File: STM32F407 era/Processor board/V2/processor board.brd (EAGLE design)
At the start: 61.4 x 43.5 mm, 45 parts, among them IC1 REG1117, U2 MAX13052ESA+, X2 057-010-1, Y1 25 MHz, Y2 32.768KHz

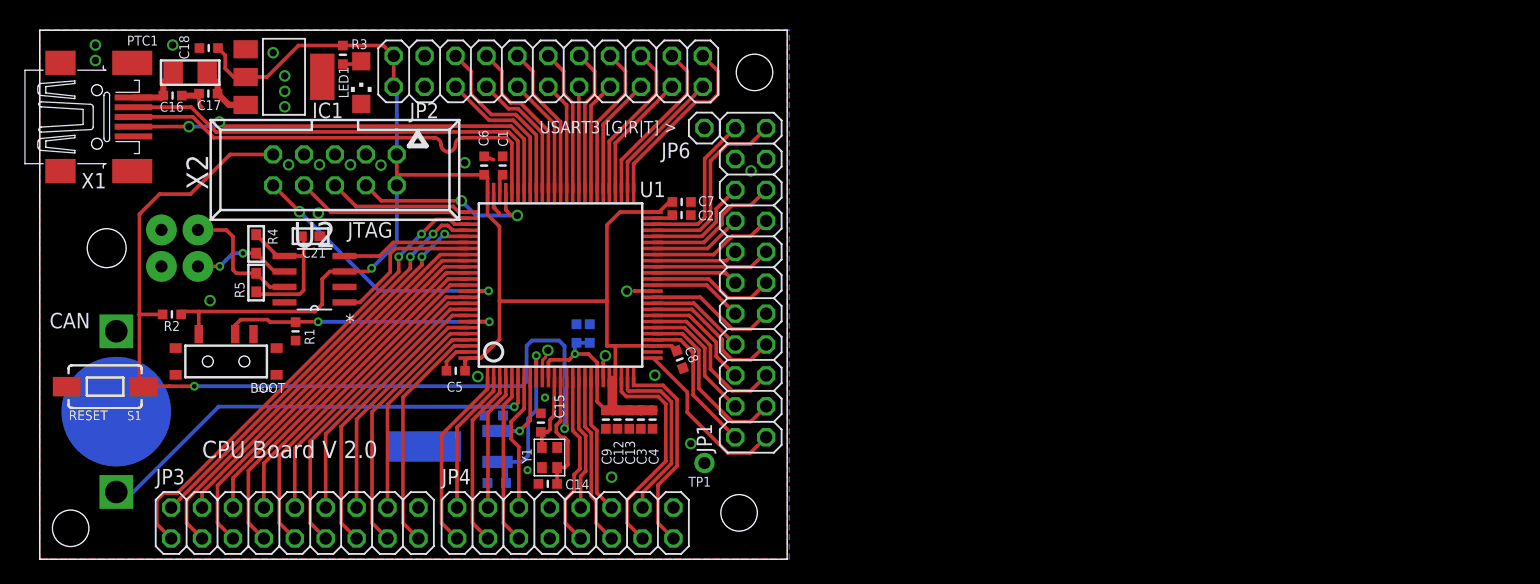
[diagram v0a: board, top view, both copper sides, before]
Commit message: more final board prepping for production
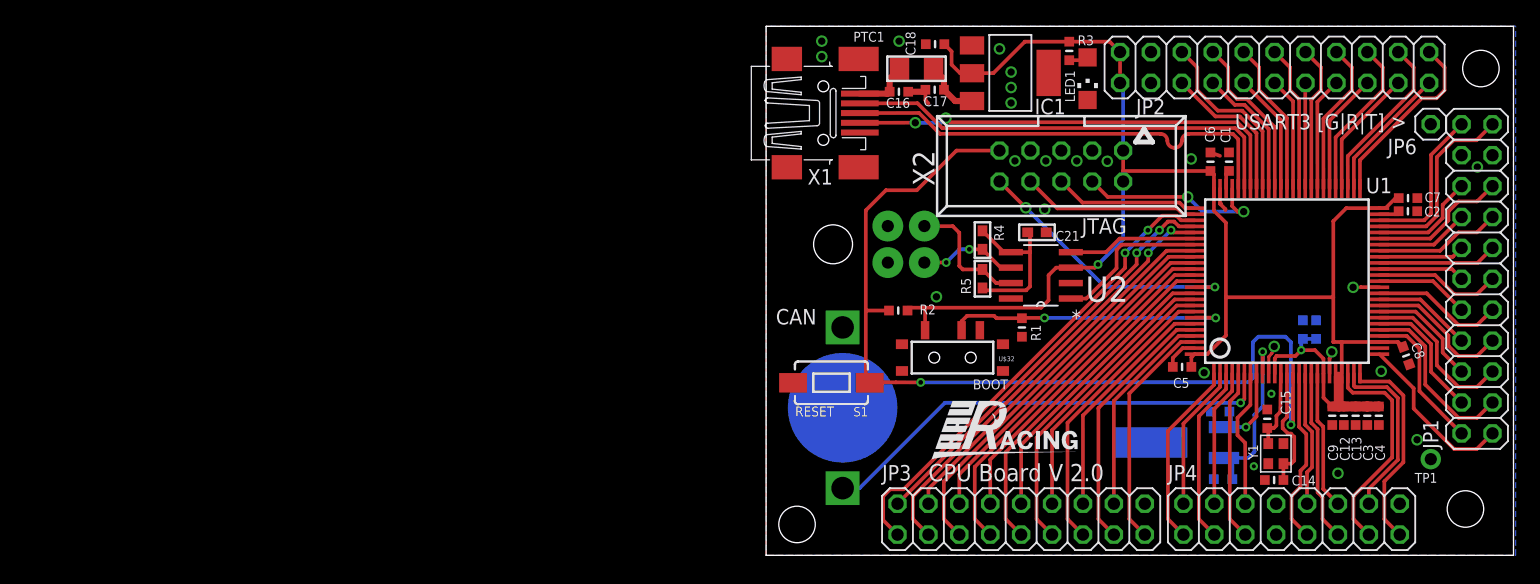
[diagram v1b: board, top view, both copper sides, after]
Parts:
- moved C10 59.7 mm to (103.8, 18.9)
- moved C11 59.7 mm to (104.9, 18.9)
- moved C12 59.7 mm to (107.2, 11.8)
- moved C13 59.7 mm to (108.1, 11.8)
- moved C18 59.7 mm to (73.6, 42.3)
- moved C19 59.7 mm to (97.0, 12.1)
- moved C2 59.7 mm to (112.4, 28.6)
- moved C3 59.7 mm to (109.1, 11.8)
- moved C7 59.7 mm to (112.4, 29.7)
- moved C9 59.7 mm to (106.2, 11.8)
- moved IC1 59.7 mm to (79.8, 40.0)
- moved JP1 59.7 mm to (118.1, 23.0)
- moved JP2 59.7 mm to (101.5, 40.4)
- moved BAT1 59.7 mm to (66.0, 12.4)
- moved C1 59.7 mm to (97.7, 32.7)
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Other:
- board text removed: "Henrik Jensen Jakob Jensen JesperJørgensen Peter Reichwald"
